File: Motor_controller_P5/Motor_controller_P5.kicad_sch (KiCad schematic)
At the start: 49 parts, among them J10 Vcc, J11 Motor ELEVATION, J3 Conn_01x04_Pin, J4 Encoder Azimtuh, J6 Home_azi, J7 Home_ele, J8 Motor AZI, J9 Barrel input, U1 L298N, U2 ESP32-DevKitC, U3 LM7805_TO220

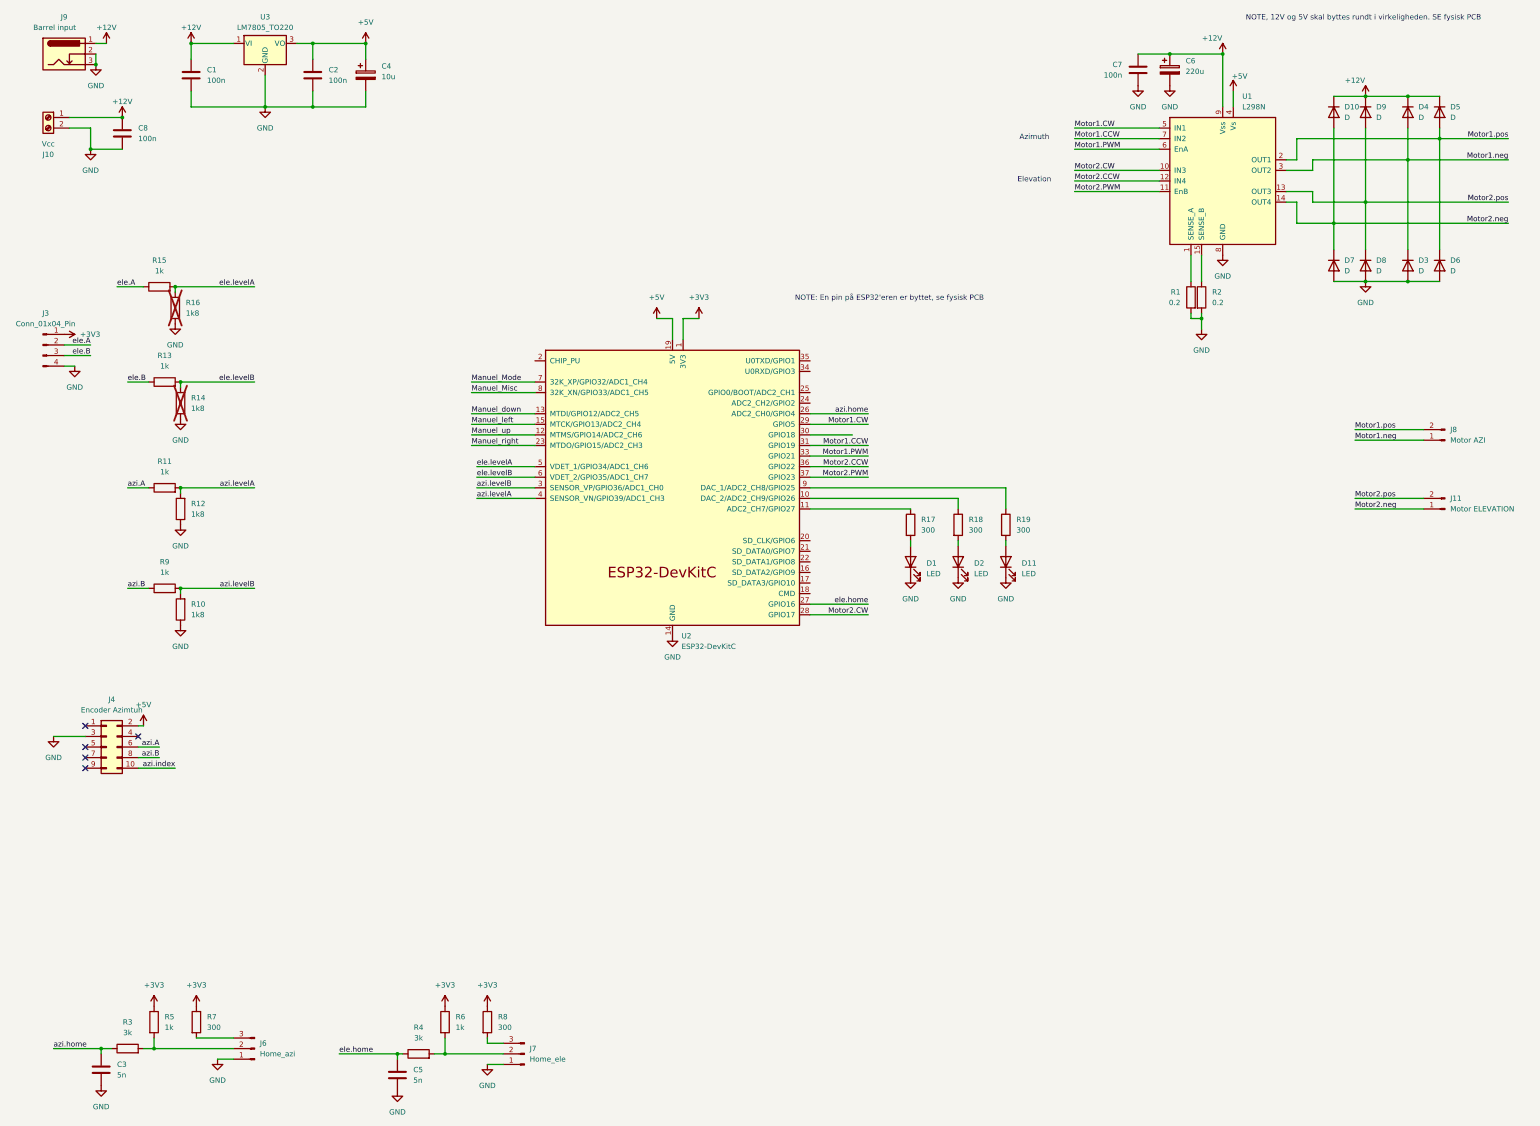
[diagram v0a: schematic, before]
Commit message: Flottede lige schematic
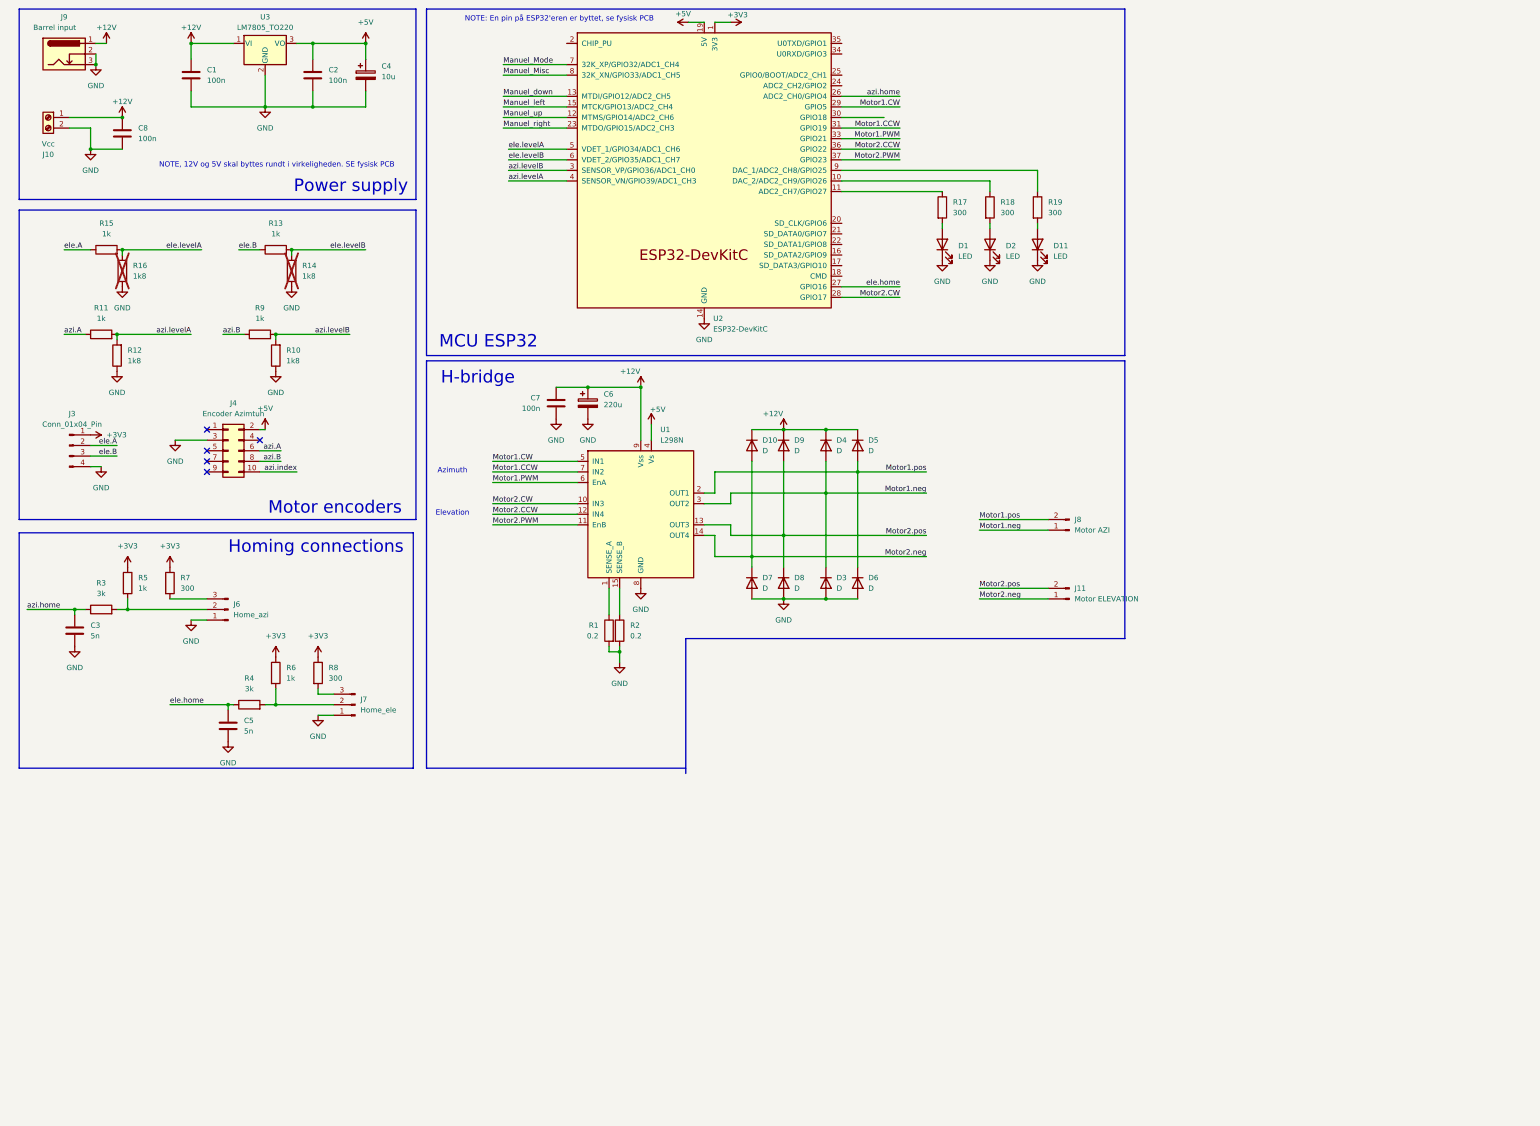
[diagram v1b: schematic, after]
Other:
- note added: "H-bridge"
- note added: "Homing connections"
- note added: "MCU ESP32"
- note added: "Motor encoders"
- note added: "Power supply"
- moved on the sheet: C3, C5, C6, C7, D1, D10, D11, D2, D3, D4, D5, D6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
